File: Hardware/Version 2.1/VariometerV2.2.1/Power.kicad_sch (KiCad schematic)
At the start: 34 parts, among them IC2 BQ25303JRTER, IC4 TPS22916CNYFPR, IC5 TPS73701DCQR, J8 LED_CHRG, Q1 AO3401A, Q2 AO3401A, Q3 AO3400A

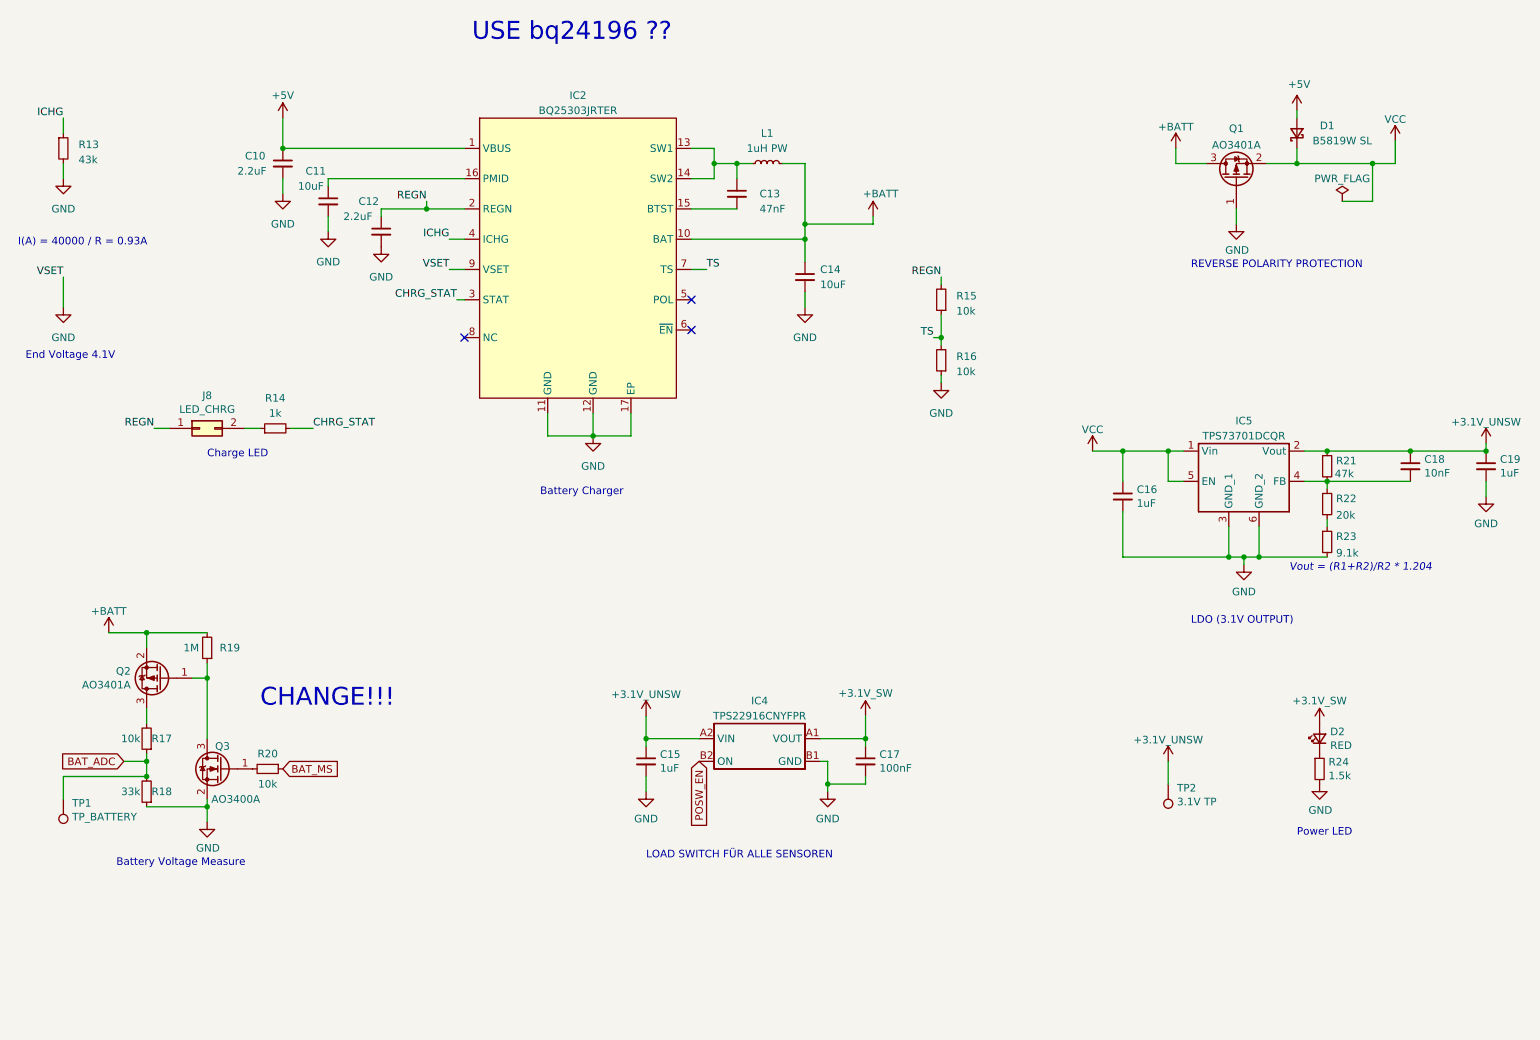
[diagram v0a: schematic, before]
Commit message: Update Schematics
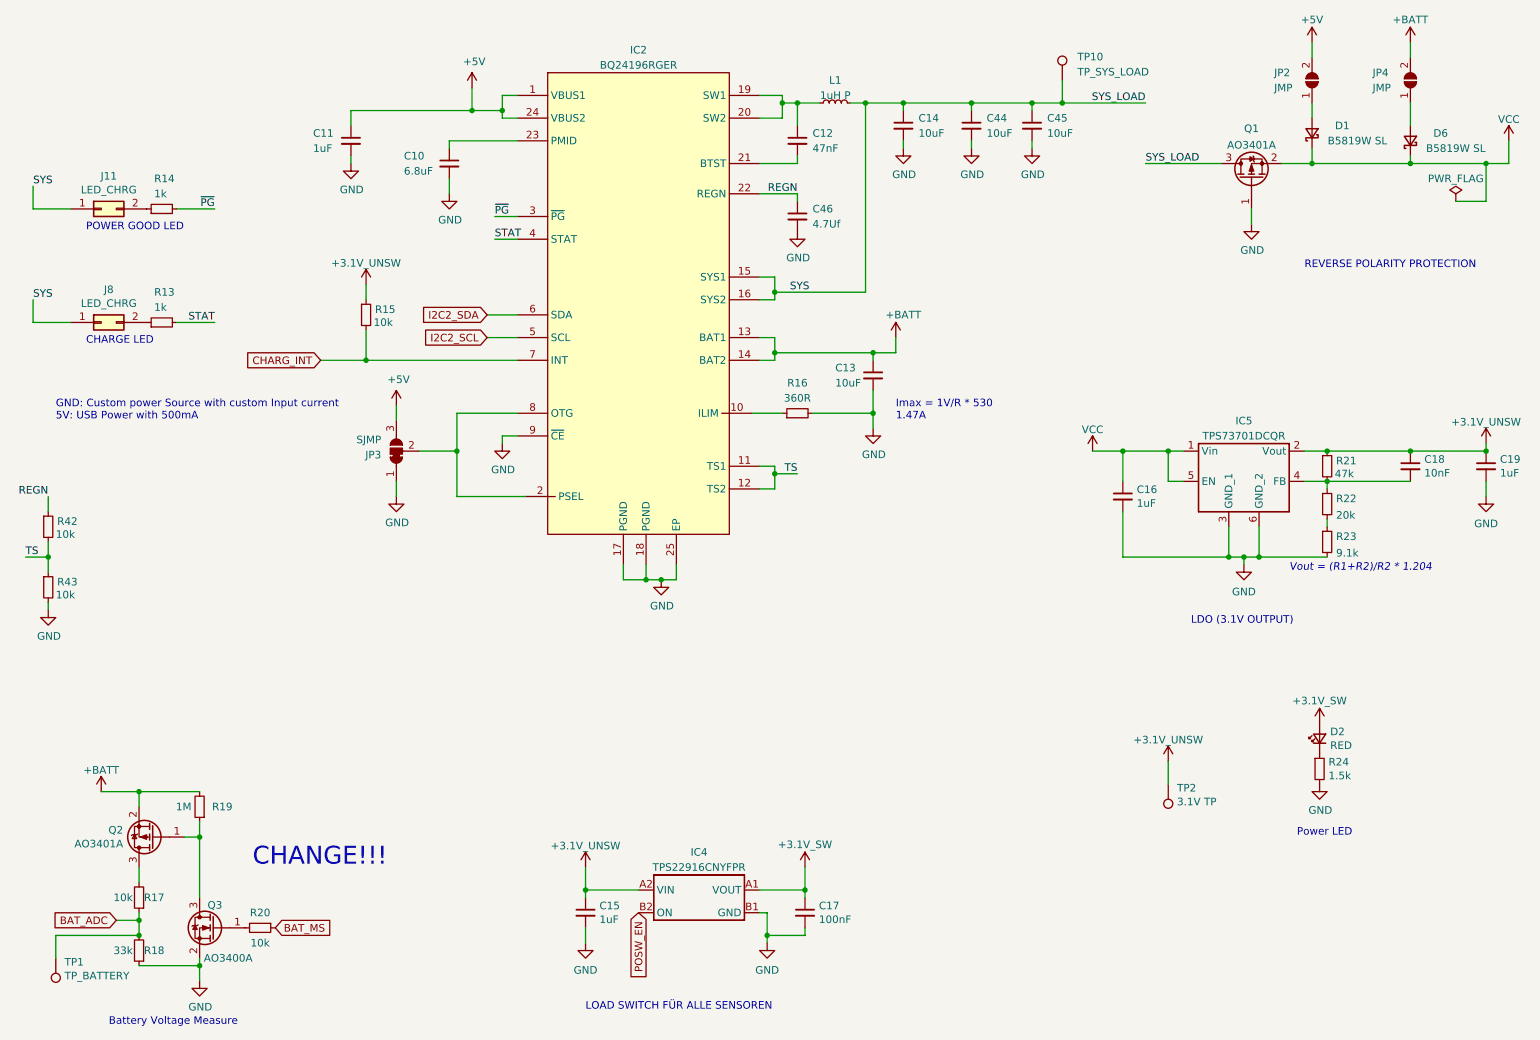
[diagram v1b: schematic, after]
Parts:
- removed IC2: BQ25303JRTER, QFN50P300X300X80-17N-D, symbol Main_LibraryVario:BQ25303JRTER
- added C44, C45: 10uF, Capacitor_SMD:C_0603_1608Metric, symbol Device:C_Small
- added C46: 4.7Uf, Capacitor_SMD:C_0603_1608Metric, symbol Device:C_Small
- added D6: B5819W SL, Diode_SMD:D_SOD-123, symbol Device:D_Schottky_Small
- added IC2: BQ24196RGER, MainLibrary:QFN50P400X400X100-25N-D, symbol Main_LibraryVario:BQ24196RGER
- added J11: LED_CHRG, Connector_PinHeader_2.54mm:PinHeader_2x01_P2.54mm_Vertical, symbol Connector_Generic:Conn_02x01
- added JP2, JP4: JMP, Jumper:SolderJumper-2_P1.3mm_Open_Pad1.0x1.5mm, symbol Jumper:SolderJumper_2_Open
- added JP3: SJMP, Jumper:SolderJumper-3_P1.3mm_Bridged12_Pad1.0x1.5mm_NumberLabels, symbol Jumper:SolderJumper_3_Bridged12
- added R42, R43: 10k, symbol Device:R_Small
- added TP10: TP_SYS_LOAD, symbol Connector:TestPoint
- C10: value 2.2uF -> 6.8uF; footprint (none) -> Capacitor_SMD:C_0603_1608Metric; JLCPCB Part # (none) -> C52923; LCSC Part # (none) -> C2345
- C11: value 10uF -> 1uF; footprint (none) -> Capacitor_SMD:C_0402_1005Metric; JLCPCB Part # (none) -> C52923; LCSC Part # (none) -> C2345
- C12: value 2.2uF -> 47nF; footprint (none) -> Capacitor_SMD:C_0603_1608Metric; JLCPCB Part # (none) -> C52923; LCSC Part # (none) -> C2345
- C13: value 47nF -> 10uF; footprint (none) -> Capacitor_SMD:C_0603_1608Metric; JLCPCB Part # (none) -> C52923; LCSC Part # (none) -> C2345
- C14: footprint (none) -> Capacitor_SMD:C_0603_1608Metric; JLCPCB Part # (none) -> C52923; LCSC Part # (none) -> C2345
- IC4: footprint SamacSys_Parts:BGA4C40P2X2_78X78X50 -> MainLibrary:BGA4C40P2X2_78X78X50
- IC5: footprint SamacSys_Parts:SOT127P706X180-6N -> MainLibrary:SOT127P706X180-6N
- J8: footprint Connector_PinHeader_2.00mm:PinHeader_2x01_P2.00mm_Vertical -> Connector_PinHeader_2.54mm:PinHeader_2x01_P2.54mm_Vertical
- L1: value 1uH PW -> 1uH P
- Q1, Q2, Q3: footprint Package_TO_SOT_SMD:SOT-23 -> (none)
- R13: value 43k -> 1k; JLCPCB Part # (none) -> C21190
- R14: JLCPCB Part # (none) -> C21190
- R15: JLCPCB Part # (none) -> C25819
- R16: value 10k -> 360R
- R17, R18, R19, R20: footprint Resistor_SMD:R_0402_1005Metric -> (none)
- R21, R22, R23, R24: footprint Resistor_SMD:R_0603_1608Metric -> (none)
- TP1, TP2: footprint TestPoint:TestPoint_Pad_D1.5mm -> (none)
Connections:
- net ICHG is gone; now on an unnamed net: R13.1
- net +3.1V_UNSW: now also R15.1
- net +5V: now also C11.1, IC2.1 (VBUS1), IC2.24 (VBUS2), JP2.2 (B), JP3.3 (B); no longer C10.1, D1.2 (A)
- net +BATT: now also C13.1, IC2.13 (BAT1), IC2.14 (BAT2), JP4.2 (B); no longer C14.1, L1.2, Q1.3 (D)
- net GND: now also C13.2, R16.2, C44.2, C45.2, C46.2, IC2.17 (PGND), IC2.18 (PGND), IC2.25 (EP), IC2.9 (~{CE}), JP3.1 (A), R43.2; no longer C12.2, R13.2, R16.1
- net REGN: now also C46.1, IC2.22 (REGN), R42.1; no longer C12.1, J8.1 (Pin_1), R15.2
- net TS: now also IC2.11 (TS1), IC2.12 (TS2), R42.2, R43.1; no longer R15.1, R16.2
- net VCC: now also D6.1 (K)
- net at L1.1: now also C12.1, IC2.19 (SW1), IC2.20 (SW2); no longer C13.1
- net at J8.2 (Pin_2): no longer R14.1
- net CHRG_STAT renamed ~{PG}
- net ~{PG}: now also IC2.3 (~{PG})
- new net: D1.2 (A), JP2.1 (A)
- new net: J11.2 (Pin_2), R14.1
- new net: IC2.2 (PSEL), IC2.8 (OTG), JP3.2 (C)
- new net: IC2.10 (ILIM), R16.1
- new net: D6.2 (A), JP4.1 (A)
- new net: C10.1, IC2.23 (PMID)
- new net: C12.2, IC2.21 (BTST)
- new net CHARG_INT: IC2.7 (INT), R15.2
- new net I2C2_SCL: IC2.5 (SCL)
- new net I2C2_SDA: IC2.6 (SDA)
- new net STAT: IC2.4 (STAT), R13.2
- new net SYS: C14.1, C44.1, C45.1, IC2.15 (SYS1), IC2.16 (SYS2), J11.1 (Pin_1), J8.1 (Pin_1), L1.2, Q1.3 (D), TP10.1
- no-connect marks 3 -> 0
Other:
- note added: "CHARGE LED"
- note added: "GND: Custom power Source with custom Input current 5V: USB Power with 500mA"
- note added: "Imax = 1V/R * 530 1.47A"
- note added: "POWER GOOD LED"
- note removed: "Battery Charger"
- note removed: "Charge LED"
- note removed: "End Voltage 4.1V"
- note removed: "I(A) = 40000 / R = 0.93A"
- note removed: "USE bq24196 ??"
- moved on the sheet: C15, C17, D1, IC4, Q1, Q2, Q3, R17, R18, R19, R20, TP1

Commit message: Working on PCB
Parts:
- Q1, Q2, Q3: footprint (none) -> Package_TO_SOT_SMD:SOT-23
- R13, R14, R15, R16, R21, R22, R23, R24, R42, R43: footprint (none) -> Resistor_SMD:R_0603_1608Metric
- R17, R18, R19, R20: footprint (none) -> Resistor_SMD:R_0402_1005Metric
- TP1, TP10, TP2: footprint (none) -> TestPoint:TestPoint_Pad_D1.5mm
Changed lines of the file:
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@@
       (effects (font (size 1.27 1.27)) (justify left))
     )
-    (property "Footprint" "" (at 49.53 175.895 0)
+    (property "Footprint" "Package_TO_SOT_SMD:SOT-23" (at 49.53 175.895 0)
       (effects (font (size 1.27 1.27) italic) (justify left) hide)
     )
@@
       (effects (font (size 1.27 1.27)))
     )
-    (property "Footprint" "" (at 62.23 173.99 0)
+    (property "Footprint" "Resistor_SMD:R_0402_1005Metric" (at 62.23 173.99 0)
       (effects (font (size 1.27 1.27)) hide)
     )
@@
       (effects (font (size 1.27 1.27)) (justify left))
     )
-    (property "Footprint" "" (at 80.01 71.12 0)
+    (property "Footprint" "Resistor_SMD:R_0603_1608Metric" (at 80.01 71.12 0)
       (effects (font (size 1.27 1.27)) hide)
     )
@@
       (effects (font (size 1.27 1.27)))
     )
-    (property "Footprint" "" (at 41.91 168.91 0)
+    (property "Footprint" "Resistor_SMD:R_0402_1005Metric" (at 41.91 168.91 0)
       (effects (font (size 1.27 1.27)) hide)
     )
@@
       (effects (font (size 1.27 1.27)) (justify right))
     )
-    (property "Footprint" "" (at 209.55 149.86 0)
+    (property "Footprint" "TestPoint:TestPoint_Pad_D1.5mm" (at 209.55 149.86 0)
       (effects (font (size 1.27 1.27)) hide)
     )
@@
       (effects (font (size 1.27 1.27)) (justify left))
     )
-    (property "Footprint" "" (at 26.67 106.68 0)
+    (property "Footprint" "Resistor_SMD:R_0603_1608Metric" (at 26.67 106.68 0)
       (effects (font (size 1.27 1.27)) hide)
     )
@@
       (effects (font (size 1.27 1.27)) (justify right))
     )
-    (property "Footprint" "" (at 45.72 72.39 0)
+    (property "Footprint" "Resistor_SMD:R_0603_1608Metric" (at 45.72 72.39 0)
       (effects (font (size 1.27 1.27)) hide)
     )
@@
       (effects (font (size 1.27 1.27)) (justify left))
     )
-    (property "Footprint" "" (at 241.3 102.87 0)
+    (property "Footprint" "Resistor_SMD:R_0603_1608Metric" (at 241.3 102.87 0)
       (effects (font (size 1.27 1.27)) hide)
     )
@@
       (effects (font (size 1.27 1.27)))
     )
-    (property "Footprint" "" (at 41.91 177.8 0)
+    (property "Footprint" "Resistor_SMD:R_0402_1005Metric" (at 41.91 177.8 0)
       (effects (font (size 1.27 1.27)) hide)
     )
@@
       (effects (font (size 1.27 1.27)) (justify left))
     )
-    (property "Footprint" "" (at 26.67 116.84 0)
+    (property "Footprint" "Resistor_SMD:R_0603_1608Metric" (at 26.67 116.84 0)
       (effects (font (size 1.27 1.27)) hide)
     )
@@
       (effects (font (size 1.27 1.27)) (justify right))
     )
-    (property "Footprint" "" (at 45.72 53.34 0)
+    (property "Footprint" "Resistor_SMD:R_0603_1608Metric" (at 45.72 53.34 0)
       (effects (font (size 1.27 1.27)) hide)
     )
@@
       (effects (font (size 1.27 1.27)))
     )
-    (property "Footprint" "" (at 152.4 87.63 0)
+    (property "Footprint" "Resistor_SMD:R_0603_1608Metric" (at 152.4 87.63 0)
       (effects (font (size 1.27 1.27)) hide)
     )
@@
       (effects (font (size 1.27 1.27)) (justify left))
     )
-    (property "Footprint" "" (at 241.3 109.22 0)
+    (property "Footprint" "Resistor_SMD:R_0603_1608Metric" (at 241.3 109.22 0)
       (effects (font (size 1.27 1.27)) hide)
     )
@@
       (effects (font (size 1.27 1.27)) (justify left))
     )
-    (property "Footprint" "" (at 39.37 156.845 0)
+    (property "Footprint" "Package_TO_SOT_SMD:SOT-23" (at 39.37 156.845 0)
       (effects (font (size 1.27 1.27) italic) (justify left) hide)
     )
@@
       (effects (font (size 1.27 1.27)) (justify right))
     )
-    (property "Footprint" "" (at 22.86 179.07 0)
+    (property "Footprint" "TestPoint:TestPoint_Pad_D1.5mm" (at 22.86 179.07 0)
       (effects (font (size 1.27 1.27)) hide)
     )
@@
       (effects (font (size 1.27 1.27)) (justify left))
     )
-    (property "Footprint" "" (at 240.03 147.32 0)
+    (property "Footprint" "Resistor_SMD:R_0603_1608Metric" (at 240.03 147.32 0)
       (effects (font (size 1.27 1.27)) hide)
     )
@@
       (effects (font (size 1.27 1.27)) (justify left))
     )
-    (property "Footprint" "" (at 241.3 96.52 0)
+    (property "Footprint" "Resistor_SMD:R_0603_1608Metric" (at 241.3 96.52 0)
       (effects (font (size 1.27 1.27)) hide)
     )
@@
       (effects (font (size 1.27 1.27)))
     )
-    (property "Footprint" "" (at 230.505 43.18 0)
+    (property "Footprint" "Package_TO_SOT_SMD:SOT-23" (at 230.505 43.18 0)
       (effects (font (size 1.27 1.27) italic) (justify left) hide)
     )
@@
       (effects (font (size 1.27 1.27)) (justify left))
     )
-    (property "Footprint" "" (at 201.93 31.75 0)
+    (property "Footprint" "TestPoint:TestPoint_Pad_D1.5mm" (at 201.93 31.75 0)
       (effects (font (size 1.27 1.27)) hide)
     )
@@
       (effects (font (size 1.27 1.27)))
     )
-    (property "Footprint" "" (at 52.07 153.67 0)
-      (effects (font (size 1.27 1.27)) hide)
-    )
+    (property "Footprint" "Resistor_SMD:R_0402_1005Metric" (at 52.07 153.67 0)
+      (effects (font (size 1.27 1.27)) hide)
+    )
